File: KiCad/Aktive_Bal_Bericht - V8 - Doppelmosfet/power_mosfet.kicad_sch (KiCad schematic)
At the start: 124 parts, among them J15 Screw_Terminal_01x03, J16 Screw_Terminal_01x03, J17 Screw_Terminal_01x03, J18 Screw_Terminal_01x03, J19 Screw_Terminal_01x03, J20 Screw_Terminal_01x03, Q10 Q_Dual_NMOS_G1S2G2D2S1D1, Q11 Q_Dual_NMOS_G1S2G2D2S1D1, Q12 Q_Dual_NMOS_G1S2G2D2S1D1, Q13 Q_Dual_NMOS_G1S2G2D2S1D1, Q14 Q_Dual_NMOS_G1S2G2D2S1D1, Q15 Q_Dual_NMOS_G1S2G2D2S1D1, Q16 Q_Dual_NMOS_G1S2G2D2S1D1, Q17 Q_Dual_NMOS_G1S2G2D2S1D1, Q18 Q_Dual_NMOS_G1S2G2D2S1D1, Q19 Q_Dual_NMOS_G1S2G2D2S1D1, Q2 Q_Dual_NMOS_G1S2G2D2S1D1, Q20 Q_Dual_NMOS_G1S2G2D2S1D1, Q21 Q_Dual_NMOS_G1S2G2D2S1D1, Q22 Q_Dual_NMOS_G1S2G2D2S1D1, Q23 Q_Dual_NMOS_G1S2G2D2S1D1, Q24 Q_Dual_NMOS_G1S2G2D2S1D1, Q25 Q_Dual_NMOS_G1S2G2D2S1D1, Q26 Q_Dual_NMOS_G1S2G2D2S1D1, Q27 Q_Dual_NMOS_G1S2G2D2S1D1, Q28 Q_Dual_NMOS_G1S2G2D2S1D1, Q29 Q_Dual_NMOS_G1S2G2D2S1D1, Q3 Q_Dual_NMOS_G1S2G2D2S1D1, Q30 Q_Dual_NMOS_G1S2G2D2S1D1, Q31 Q_Dual_NMOS_G1S2G2D2S1D1, Q32 Q_Dual_NMOS_G1S2G2D2S1D1, Q33 Q_Dual_NMOS_G1S2G2D2S1D1, Q4 Q_Dual_NMOS_G1S2G2D2S1D1, Q5 Q_Dual_NMOS_G1S2G2D2S1D1, Q6 Q_Dual_NMOS_G1S2G2D2S1D1, Q7 Q_Dual_NMOS_G1S2G2D2S1D1, Q8 Q_Dual_NMOS_G1S2G2D2S1D1, Q9 Q_Dual_NMOS_G1S2G2D2S1D1, U10 LTV-847S, U11 LTV-847S, U12 LTV-847S, U13 LTV-847S

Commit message: mosfets verkabelt elkos getauscht
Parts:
- added unit 2 of Q2
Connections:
- net Cell16: now also Q2.4 (D); no longer Q2.4 (D)
- net Gate_HIGH_B16: now also Q2.3 (G); no longer Q2.3 (G)
- net at Q2.5 (S): now also Q2.2 (S); no longer Q2.2 (S)

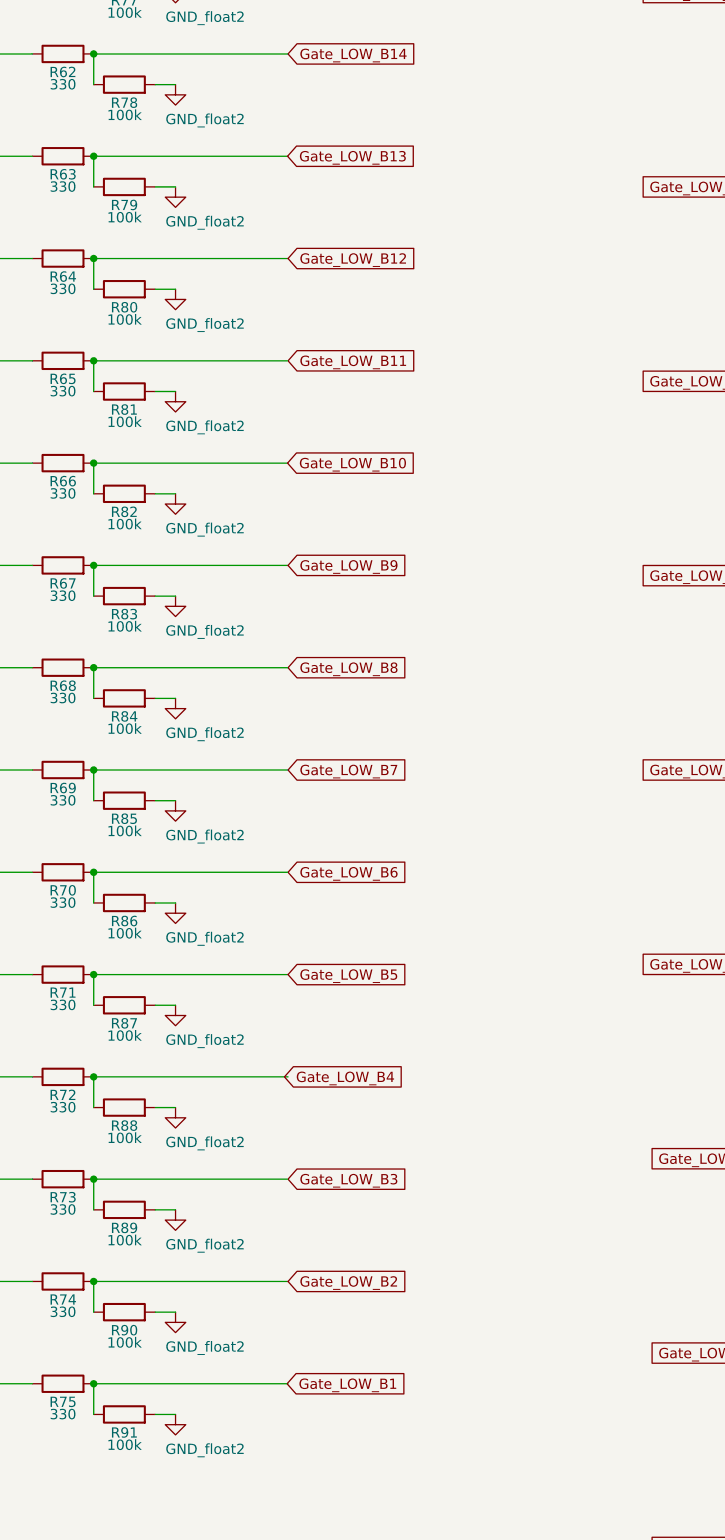
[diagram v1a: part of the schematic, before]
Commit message: neuu
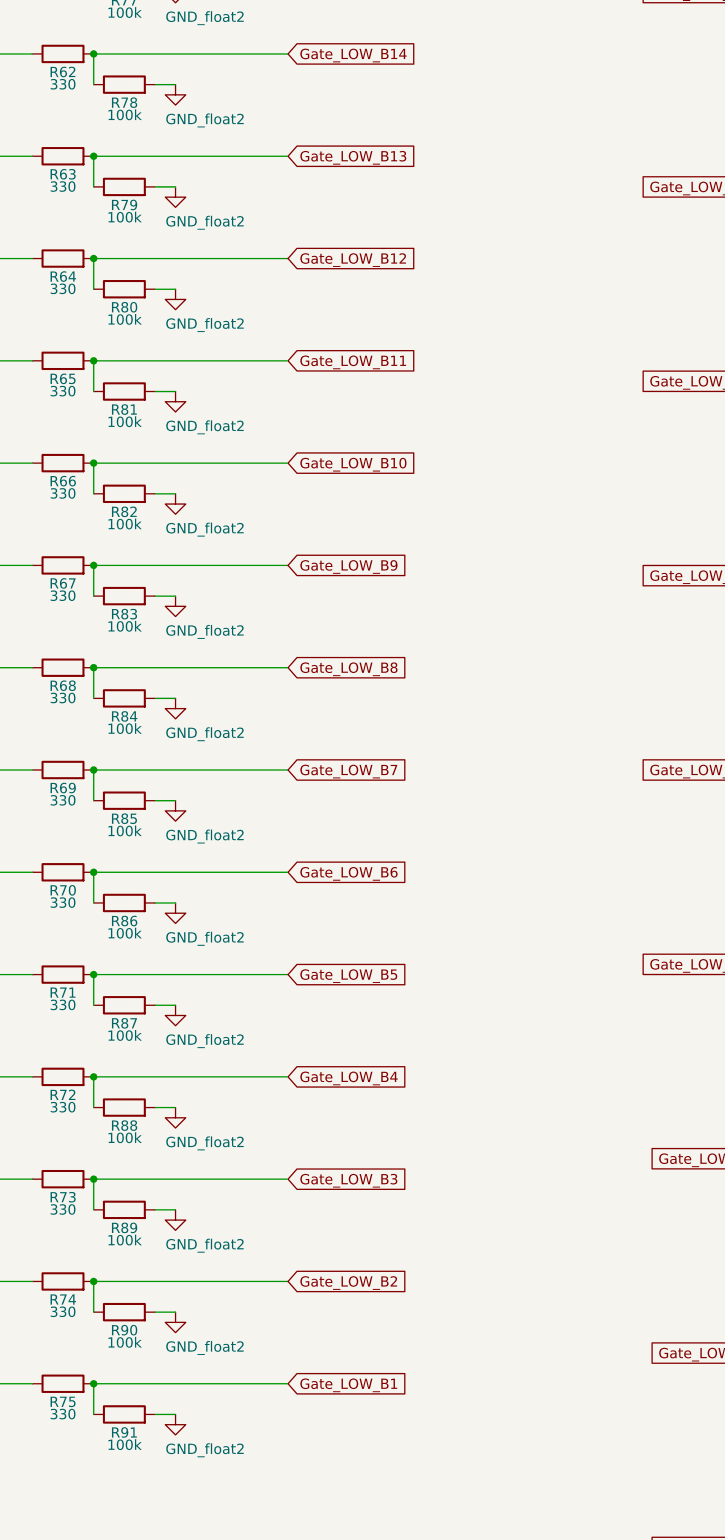
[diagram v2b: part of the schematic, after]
